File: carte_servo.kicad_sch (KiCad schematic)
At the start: 37 parts, among them J16 Conn_01x04_Male, J17 Conn_01x04_Male, J2 Conn_02x04_Top_Bottom, J24 Conn_LEDs, P1 USB_C_Plug_USB2.0, SW1 CK_KMS2xxG, U1 XGZP6897D_differential_pressu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, U2 XGZP6897D_differential_pressu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, U6 SN65HVD230, U7 LD1117S33TR_SOT223, U8 ESP32-S3-WROOM-1

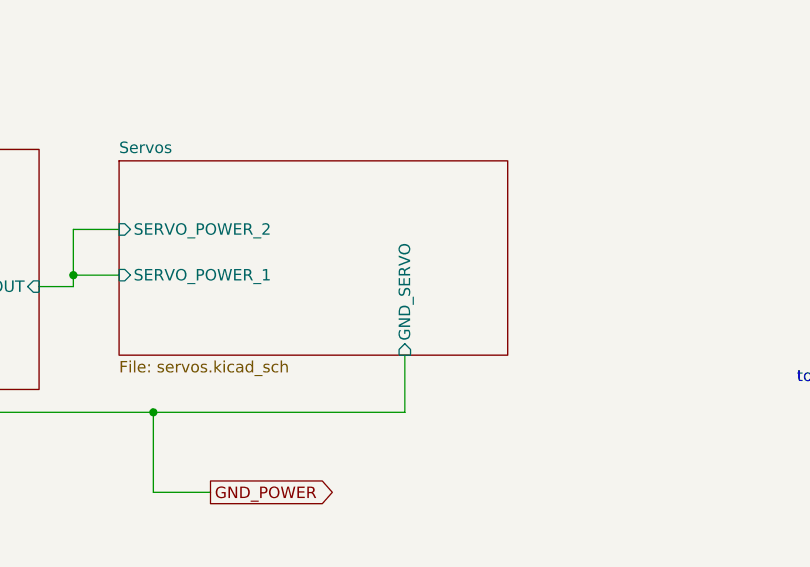
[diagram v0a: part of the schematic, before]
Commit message: small stuff
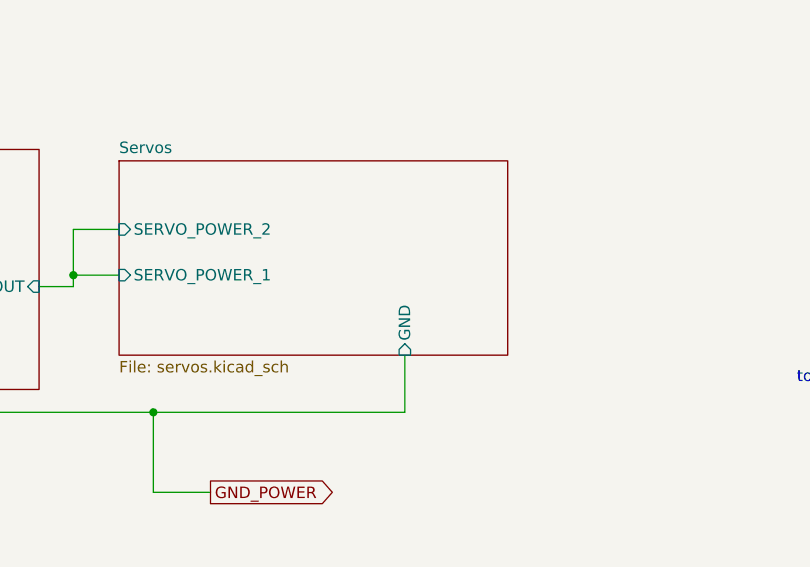
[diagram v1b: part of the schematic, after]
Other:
- sheet Servos ports: added GND; removed GND_SERVO
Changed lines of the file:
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@@
 	(label "Pressure_2"
 		(at 83.82 127 180)
-		(fields_autoplaced yes)
 		(effects
 			(font
@@
 	(label "Pressure_1"
 		(at 82.55 100.33 180)
-		(fields_autoplaced yes)
 		(effects
 			(font
@@
 			)
 		)
-		(pin "GND_SERVO" input
-			(at 257.81 46.99 270)
+		(pin "SERVO_POWER_1" input
+			(at 226.06 38.1 180)
 			(effects
 				(font
@@
 			)
 		)
-		(pin "SERVO_POWER_1" input
-			(at 226.06 38.1 180)
+		(pin "GND" input
+			(at 257.81 46.99 270)
 			(effects
 				(font
